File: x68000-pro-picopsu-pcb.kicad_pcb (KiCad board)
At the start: 2 copper layers, 209 x 98 mm, 27 parts, among them J1 Fan Header, J2 Screw_Terminal_01x07, J3 Screw_Terminal_01x07, J4 PicoPSU, U1 74LS04

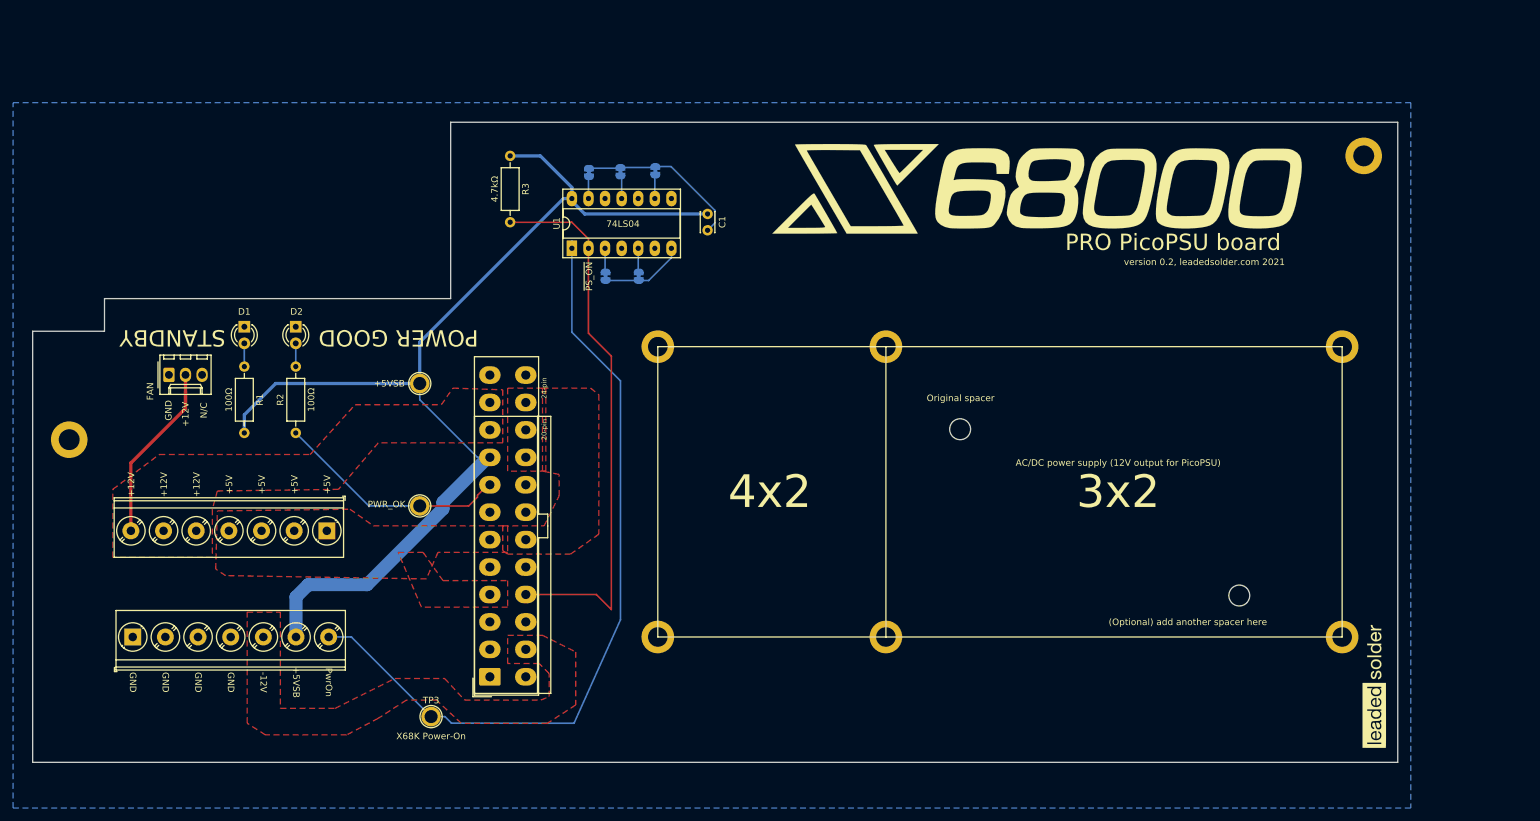
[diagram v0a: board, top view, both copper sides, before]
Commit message: Update README
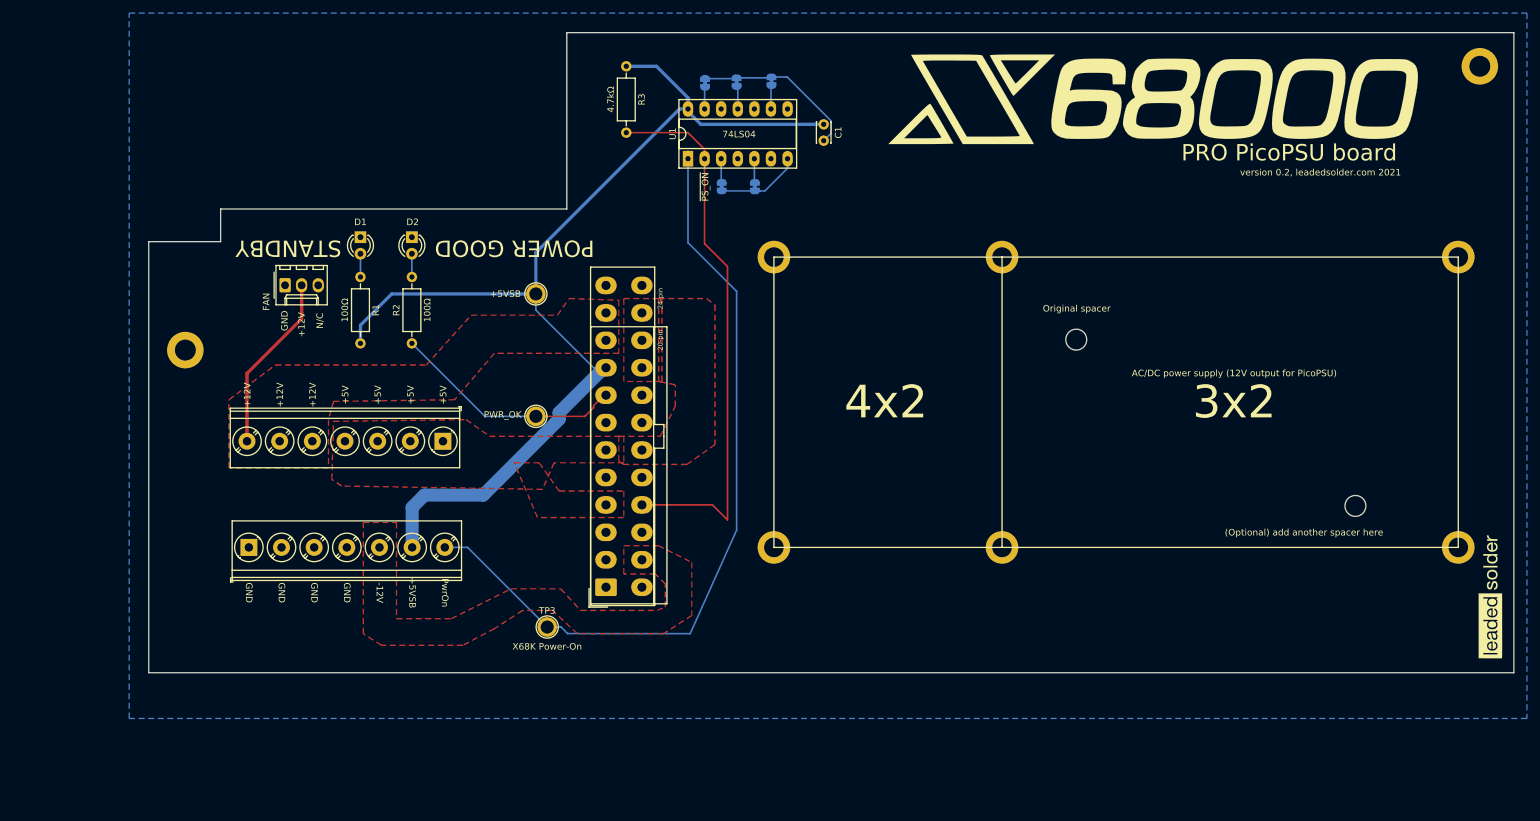
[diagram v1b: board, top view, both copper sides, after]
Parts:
- moved C1 22.5 mm to (142.1, 52.3)
- moved CONV_1 22.5 mm to (239.3, 117.1)
- moved G*** 22.5 mm to (218.2, 131.1)
- moved G*** 22.5 mm to (192.6, 48.5)
- moved G*** 22.5 mm to (244.2, 124.7)
- moved J4 22.5 mm to (108.8, 123.2)
- moved JP1 22.5 mm to (126.5, 61.9)
- moved JP2 22.5 mm to (131.6, 61.9)
- moved JP3 22.5 mm to (134.1, 45.7)
- moved JP5 22.5 mm to (124.0, 46.0)
- moved R1 22.5 mm to (71.2, 75.7)
- moved R3 22.5 mm to (111.9, 43.4)
- moved REF** 22.5 mm to (242.6, 43.4)
- moved TP3 22.5 mm to (99.8, 129.3)
- moved U1 22.5 mm to (121.3, 57.6)
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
